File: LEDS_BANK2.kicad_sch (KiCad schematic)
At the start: 76 parts, among them U12 STP16CPC26T

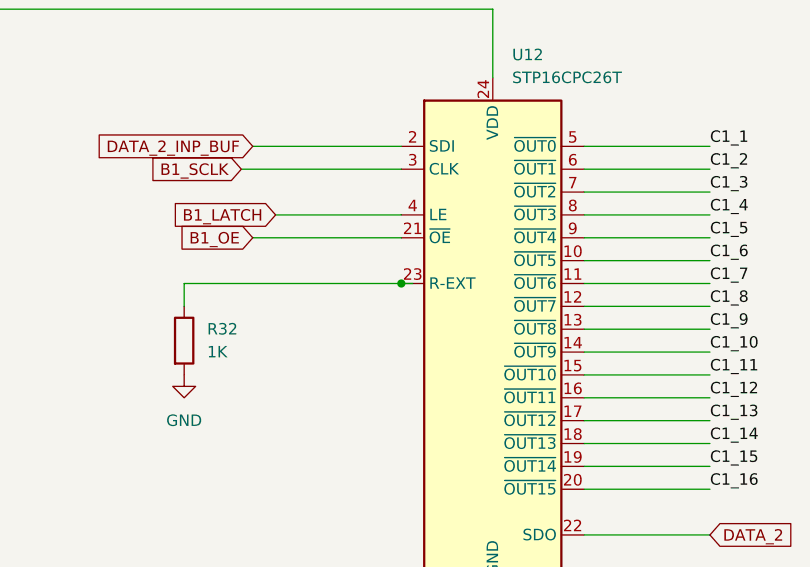
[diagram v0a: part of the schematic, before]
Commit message: sample
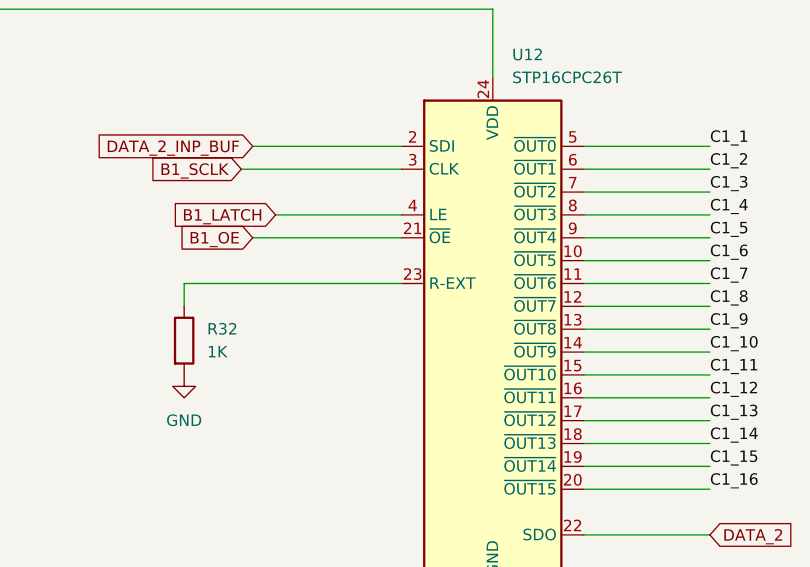
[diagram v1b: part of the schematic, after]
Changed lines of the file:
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@@
-	)
-	(junction
-		(at 82.55 158.75)
-		(diameter 0)
-		(color 0 0 0 0)
 	)
 	(junction
@@
 	(wire
 		(pts
-			(xy 82.55 158.75) (xy 83.82 158.75)
-		)
-		(stroke
-			(width 0)
-			(type default)
-		)
-	)
-	(wire
-		(pts
 			(xy 86.36 72.39) (xy 97.79 72.39)
 		)
@@
 	(wire
 		(pts
+			(xy 35.56 128.27) (xy 92.71 128.27)
+		)
+		(stroke
+			(width 0)
+			(type default)
+		)
+	)
+	(wire
+		(pts
+			(xy 102.87 143.51) (xy 116.84 143.51)
+		)
+		(stroke
+			(width 0)
+			(type default)
+		)
+	)
+	(wire
+		(pts
+			(xy 232.41 101.6) (xy 232.41 109.22)
+		)
+		(stroke
+			(width 0)
+			(type default)
+		)
+	)
+	(wire
+		(pts
+			(xy 62.23 72.39) (xy 73.66 72.39)
+		)
+		(stroke
+			(width 0)
+			(type default)
+		)
+	)
+	(wire
+		(pts
+			(xy 250.19 15.24) (xy 250.19 25.4)
+		)
+		(stroke
+			(width 0)
+			(type default)
+		)
+	)
+	(wire
+		(pts
+			(xy 147.32 101.6) (xy 147.32 109.22)
+		)
+		(stroke
+			(width 0)
+			(type default)
+		)
+	)
+	(wire
+		(pts
+			(xy 102.87 171.45) (xy 116.84 171.45)
+		)
+		(stroke
+			(width 0)
+			(type default)
+		)
+	)
+	(wire
+		(pts
+			(xy 26.67 80.01) (xy 26.67 72.39)
+		)
+		(stroke
+			(width 0)
+			(type default)
+		)
+	)
+	(wire
+		(pts
+			(xy 102.87 151.13) (xy 116.84 151.13)
+		)
+		(stroke
+			(width 0)
+			(type default)
+		)
+	)
+	(wire
+		(pts
+			(xy 110.49 15.24) (xy 110.49 24.13)
+		)
+		(stroke
+			(width 0)
+			(type default)
+		)
+	)
+	(wire
+		(pts
+			(xy 102.87 158.75) (xy 116.84 158.75)
+		)
+		(stroke
+			(width 0)
+			(type default)
+		)
+	)
+	(wire
+		(pts
+			(xy 208.28 86.36) (xy 208.28 93.98)
+		)
+		(stroke
+			(width 0)
+			(type default)
+		)
+	)
+	(wire
+		(pts
+			(xy 195.58 101.6) (xy 195.58 109.22)
+		)
+		(stroke
+			(width 0)
+			(type default)
+		)
+	)
+	(wire
+		(pts
+			(xy 160.02 31.75) (xy 160.02 39.37)
+		)
+		(stroke
+			(width 0)
+			(type default)
+		)
+	)
+	(wire
+		(pts
+			(xy 208.28 31.75) (xy 208.28 39.37)
+		)
+		(stroke
+			(width 0)
+			(type default)
+		)
+	)
+	(wire
+		(pts
+			(xy 195.58 72.39) (xy 208.28 72.39)
+		)
+		(stroke
+			(width 0)
+			(type default)
+		)
+	)
+	(wire
+		(pts
+			(xy 97.79 58.42) (xy 97.79 66.04)
+		)
+		(stroke
+			(width 0)
+			(type default)
+		)
+	)
+	(wire
+		(pts
+			(xy 134.62 46.99) (xy 134.62 50.8)
+		)
+		(stroke
+			(width 0)
+			(type default)
+		)
+	)
+	(wire
+		(pts
+			(xy 171.45 86.36) (xy 171.45 93.98)
+		)
+		(stroke
+			(width 0)
+			(type default)
+		)
+	)
+	(wire
+		(pts
+			(xy 219.71 72.39) (xy 232.41 72.39)
+		)
+		(stroke
+			(width 0)
+			(type default)
+		)
+	)
+	(wire
+		(pts
 			(xy 58.42 158.75) (xy 82.55 158.75)
 		)
 		(stroke
-			(width 0)
-			(type default)
-		)
-	)
-	(wire
-		(pts
-			(xy 35.56 128.27) (xy 92.71 128.27)
-		)
-		(stroke
-			(width 0)
-			(type default)
-		)
-	)
-	(wire
-		(pts
-			(xy 102.87 143.51) (xy 116.84 143.51)
-		)
-		(stroke
-			(width 0)
-			(type default)
-		)
-	)
-	(wire
-		(pts
-			(xy 232.41 101.6) (xy 232.41 109.22)
-		)
-		(stroke
-			(width 0)
-			(type default)
-		)
-	)
-	(wire
-		(pts
-			(xy 62.23 72.39) (xy 73.66 72.39)
-		)
-		(stroke
-			(width 0)
-			(type default)
-		)
-	)
-	(wire
-		(pts
-			(xy 250.19 15.24) (xy 250.19 25.4)
-		)
-		(stroke
-			(width 0)
-			(type default)
-		)
-	)
-	(wire
-		(pts
-			(xy 147.32 101.6) (xy 147.32 109.22)
-		)
-		(stroke
-			(width 0)
-			(type default)
-		)
-	)
-	(wire
-		(pts
-			(xy 102.87 171.45) (xy 116.84 171.45)
-		)
-		(stroke
-			(width 0)
-			(type default)
-		)
-	)
-	(wire
-		(pts
-			(xy 26.67 80.01) (xy 26.67 72.39)
-		)
-		(stroke
-			(width 0)
-			(type default)
-		)
-	)
-	(wire
-		(pts
-			(xy 102.87 151.13) (xy 116.84 151.13)
-		)
-		(stroke
-			(width 0)
-			(type default)
-		)
-	)
-	(wire
-		(pts
-			(xy 110.49 15.24) (xy 110.49 24.13)
-		)
-		(stroke
-			(width 0)
-			(type default)
-		)
-	)
-	(wire
-		(pts
-			(xy 102.87 158.75) (xy 116.84 158.75)
-		)
-		(stroke
-			(width 0)
-			(type default)
-		)
-	)
-	(wire
-		(pts
-			(xy 208.28 86.36) (xy 208.28 93.98)
-		)
-		(stroke
-			(width 0)
-			(type default)
-		)
-	)
-	(wire
-		(pts
-			(xy 195.58 101.6) (xy 195.58 109.22)
-		)
-		(stroke
-			(width 0)
-			(type default)
-		)
-	)
-	(wire
-		(pts
-			(xy 160.02 31.75) (xy 160.02 39.37)
-		)
-		(stroke
-			(width 0)
-			(type default)
-		)
-	)
-	(wire
-		(pts
-			(xy 208.28 31.75) (xy 208.28 39.37)
-		)
-		(stroke
-			(width 0)
-			(type default)
-		)
-	)
-	(wire
-		(pts
-			(xy 195.58 72.39) (xy 208.28 72.39)
-		)
-		(stroke
-			(width 0)
-			(type default)
-		)
-	)
-	(wire
-		(pts
-			(xy 97.79 58.42) (xy 97.79 66.04)
-		)
-		(stroke
-			(width 0)
-			(type default)
-		)
-	)
-	(wire
-		(pts
-			(xy 134.62 46.99) (xy 134.62 50.8)
-		)
-		(stroke
-			(width 0)
-			(type default)
-		)
-	)
-	(wire
-		(pts
-			(xy 171.45 86.36) (xy 171.45 93.98)
-		)
-		(stroke
-			(width 0)
-			(type default)
-		)
-	)
-	(wire
-		(pts
-			(xy 219.71 72.39) (xy 232.41 72.39)
-		)
-		(stroke
